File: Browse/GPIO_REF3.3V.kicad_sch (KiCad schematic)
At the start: 14 parts, among them IC5 TPS2121RUXT

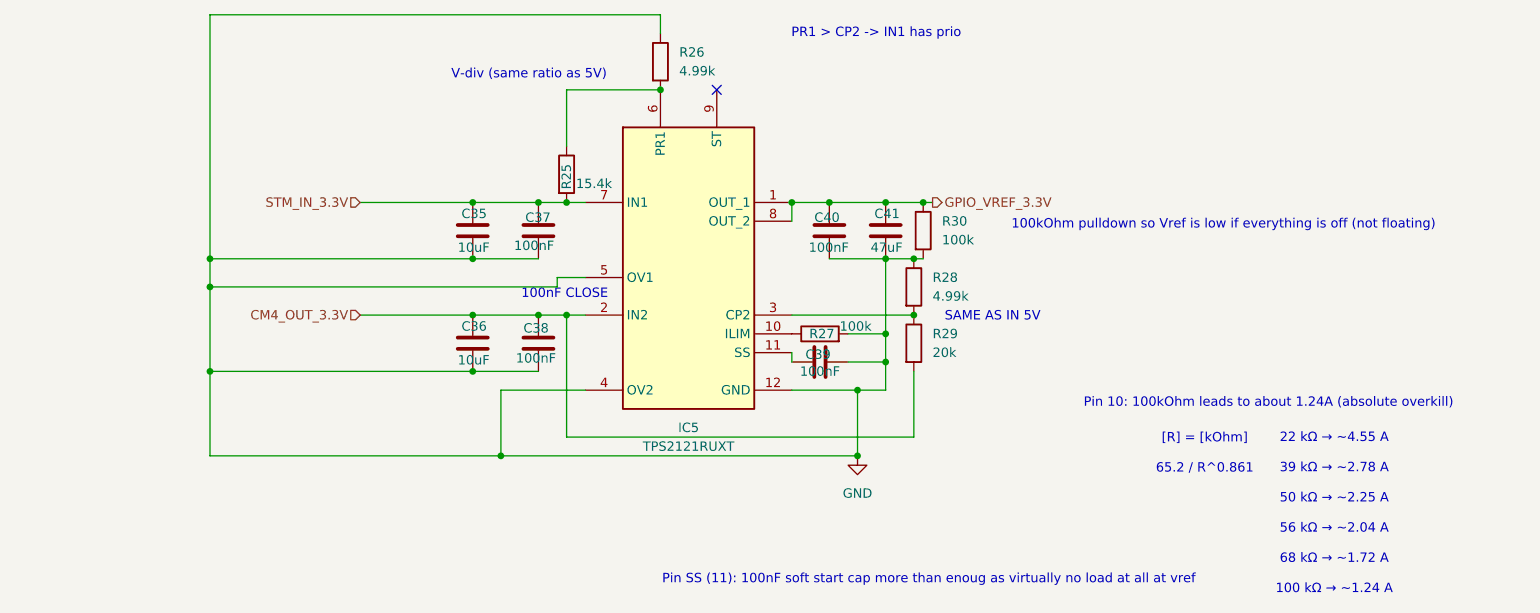
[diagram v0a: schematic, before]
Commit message: Deploying to gh-pages from @ Nautilus-UUV/nautilus-mainboard-PCB@f1dd6ce1e57c066b805694b10777c719502cca87 🚀
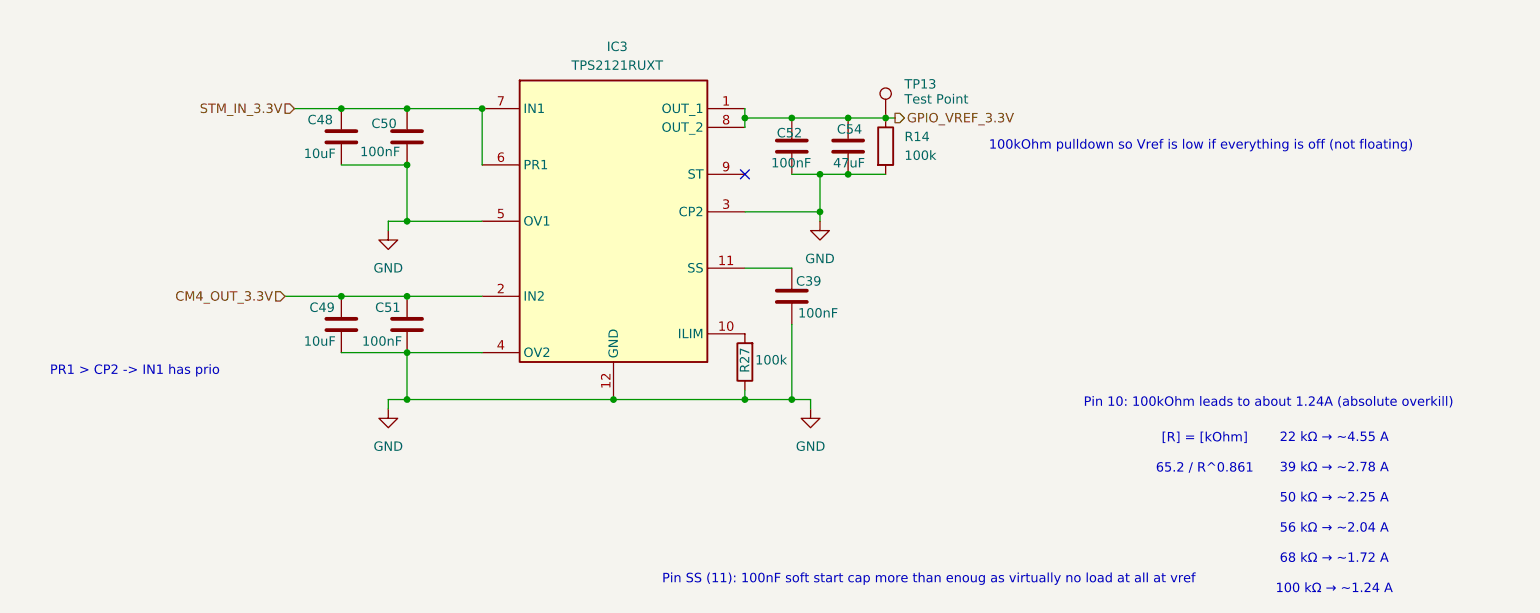
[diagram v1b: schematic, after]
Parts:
- removed C35, C36: 10uF, Capacitor_SMD:C_1210_3225Metric, symbol #dzdb:s_cap/C-MUR-GRM32EC72A106KE05
- removed C37, C38, C40: 100nF, Capacitor_SMD:C_0603_1608Metric, symbol #dzdb:g_cap/C-100n-0603
- removed C41: 47uF, Capacitor_SMD:C_0805_2012Metric, symbol #dzdb:s_cap/C-MUR-GRM21BR61A476ME15
- removed IC5: TPS2121RUXT, dz_dio:TI_Switchover_TPS2121RUXT, symbol #dzdb:s_misc/TEXA-595-TPS2121RUXT
- removed R25: 15.4k, Resistor_SMD:R_0603_1608Metric, symbol #dzdb:g_res/R-15.4k-0603
- removed R26, R28: 4.99k, Resistor_SMD:R_0603_1608Metric, symbol #dzdb:g_res/R-4.99k-0603
- removed R29: 20k, Resistor_SMD:R_0603_1608Metric, symbol #dzdb:g_res/R-20k-0603
- removed R30: 100k, Resistor_SMD:R_0603_1608Metric, symbol #dzdb:g_res/R-100k-0603
- added C48, C49: 10uF, Capacitor_SMD:C_1210_3225Metric, symbol #dzdb:s_cap/C-MUR-GRM32EC72A106KE05
- added C50, C51, C52: 100nF, Capacitor_SMD:C_0603_1608Metric, symbol #dzdb:g_cap/C-100n-0603
- added C54: 47uF, Capacitor_SMD:C_0805_2012Metric, symbol #dzdb:s_cap/C-MUR-GRM21BR61A476ME15
- added IC3: TPS2121RUXT, dz_dio:TI_Switchover_TPS2121RUXT, symbol #dzdb:s_misc/TEXA-595-TPS2121RUXT
- added R14: 100k, Resistor_SMD:R_0603_1608Metric, symbol #dzdb:g_res/R-100k-0603
- added TP13: Test Point, TestPoint:TestPoint_Pad_D1.5mm, symbol #dzdb:g_mech/M-TEST-SMT_1.5mm_round
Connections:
- net CM4_OUT_3.3V: now also C49.1, C51.1, IC3.2 (IN2)
- net GND: now also C39.1, R27.1, C48.2, C49.2, C50.2, C51.2, C52.2, C54.2, IC3.12 (GND), IC3.3 (CP2), IC3.4 (OV2), IC3.5 (OV1), R14.2; no longer C39.2, R27.2
- net GPIO_VREF_3.3V: now also C52.1, C54.1, IC3.1 (OUT_1), IC3.8 (OUT_2), R14.1, TP13.1
- net STM_IN_3.3V: now also C48.1, C50.1, IC3.6 (PR1), IC3.7 (IN1)
- new net: C39.2, IC3.11 (SS)
- new net: IC3.10 (ILIM), R27.2
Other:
- note removed: "100nF CLOSE"
- note removed: "SAME AS IN 5V"
- note removed: "V-div (same ratio as 5V)"
- company: (none) -> Davide
- title: (none) -> Nautilus_Mainboard
- moved on the sheet: C39, R27
